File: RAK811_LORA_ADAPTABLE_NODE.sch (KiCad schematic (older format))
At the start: 32 parts, among them J1 Screw_Terminal_01x02, J10 Conn_01x01_Male, J11 Conn_01x01_Male, J12 Conn_01x01_Male, J13 Conn_01x01_Male, J14 Conn_01x01_Male, J15 Conn_01x01_Male, J16 Conn_01x01_Male, J17 Conn_01x01_Male, J18 Conn_01x01_Male, J19 Conn_01x01_Male, J2 Screw_Terminal_01x03, J20 Conn_01x01_Male, J21 Conn_01x01_Male, J22 Conn_01x01_Male, J23 Conn_01x01_Male, J3 Conn_01x01_Male, J4 Conn_01x01_Male, J5 Conn_01x01_Male, J6 Conn_01x01_Male, J7 Conn_Coaxial, J8 Conn_01x01_Male, J9 Conn_01x01_Male, U1 RAK811-HF

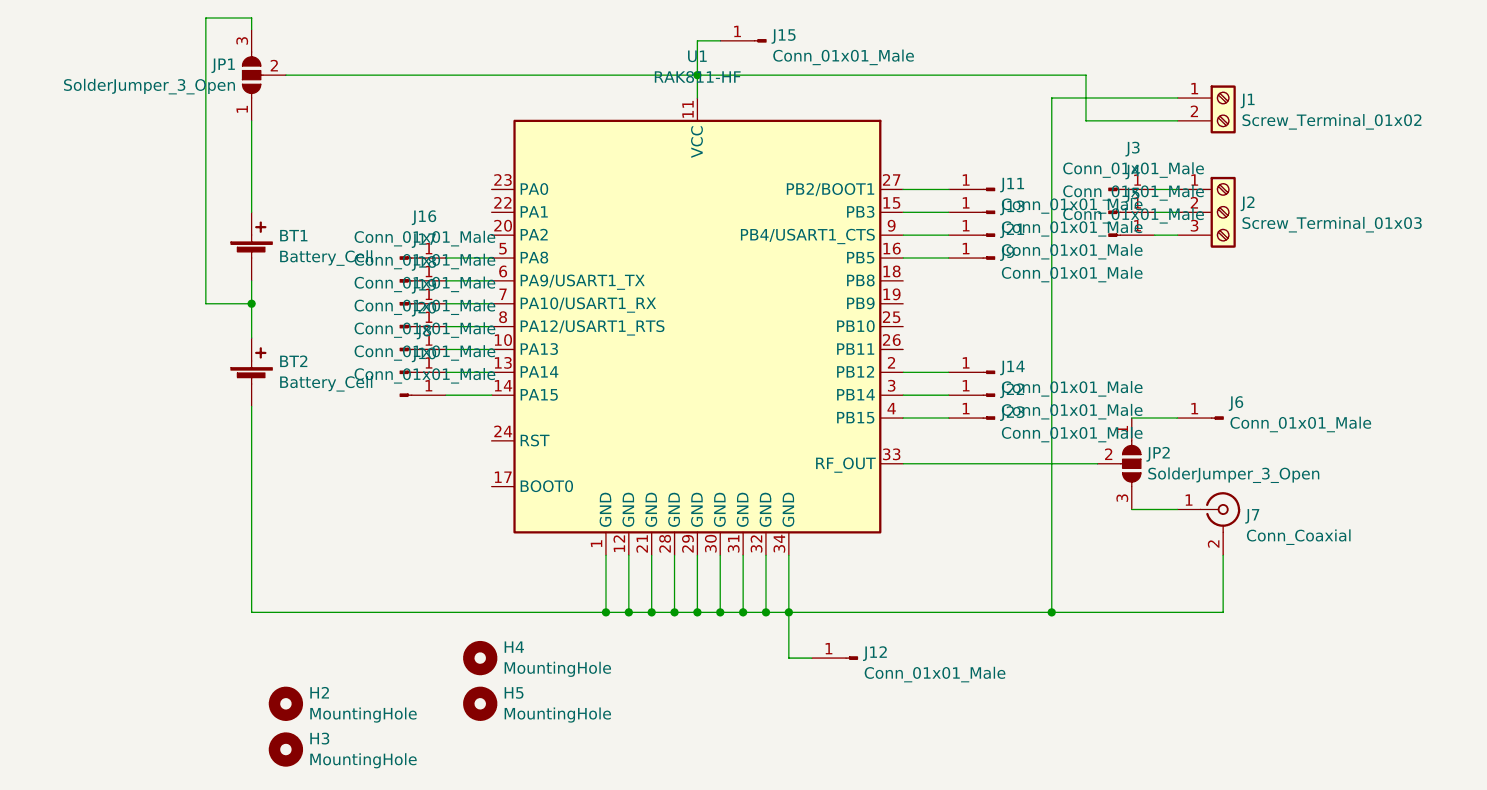
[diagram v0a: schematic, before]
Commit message: all i/o pins layout
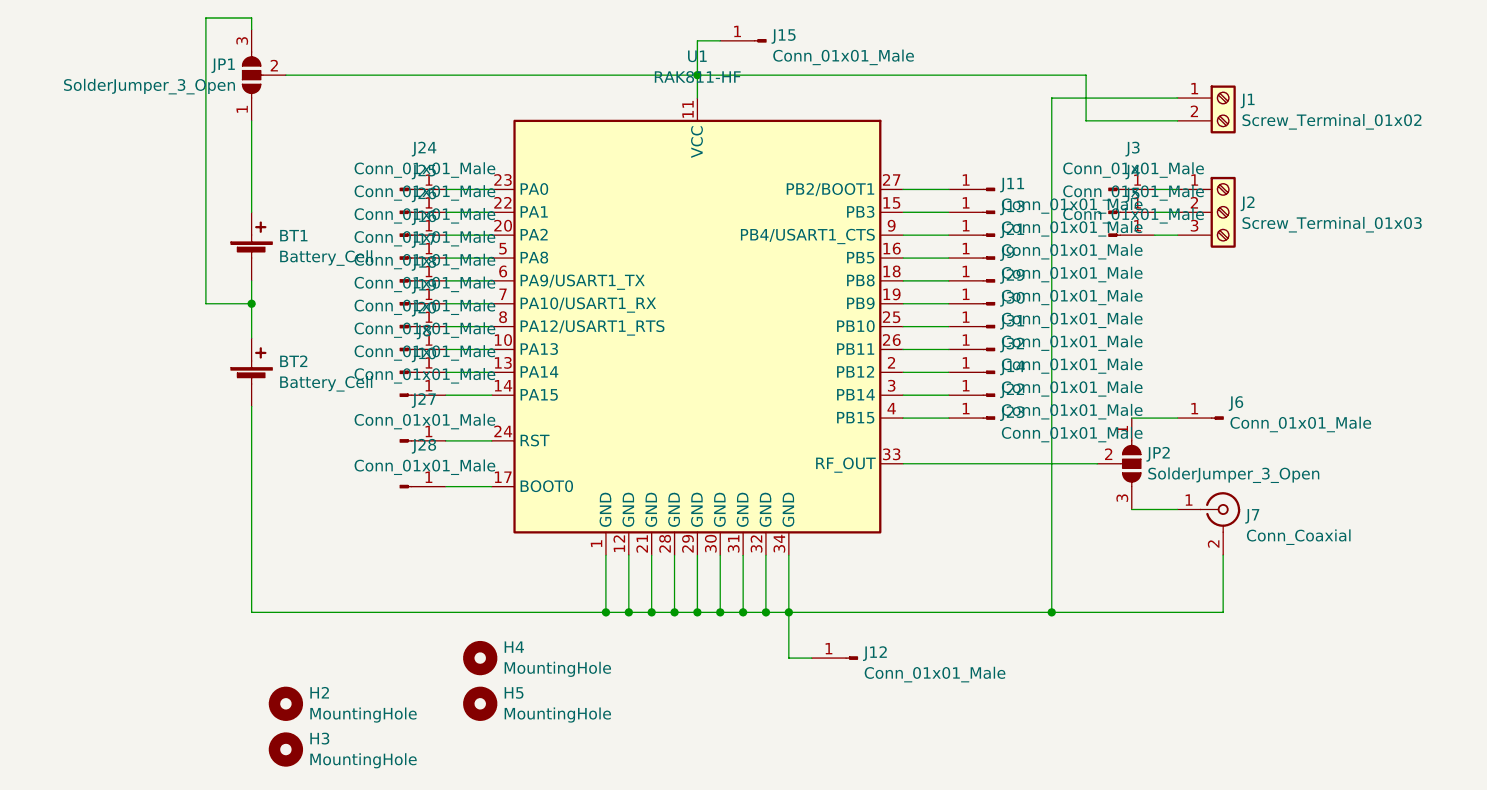
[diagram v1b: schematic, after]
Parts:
- added J24, J25, J26, J27, J28, J29, J30, J31, J32: Conn_01x01_Male, Connector_Wire:SolderWirePad_1x01_Drill0.8mm, symbol Connector:Conn_01x01_Male
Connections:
- net at U1.17 (BOOT0): now also J28.1 (Pin_1)
- net at U1.18 (PB8): now also J29.1 (Pin_1)
- net at U1.19 (PB9): now also J30.1 (Pin_1)
- net at U1.20 (PA2): now also J26.1 (Pin_1)
- net at U1.22 (PA1): now also J25.1 (Pin_1)
- net at U1.23 (PA0): now also J24.1 (Pin_1)
- net at U1.24 (RST): now also J27.1 (Pin_1)
- net at U1.25 (PB10): now also J31.1 (Pin_1)
- net at U1.26 (PB11): now also J32.1 (Pin_1)
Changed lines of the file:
@@
 Wire Wire Line
 	4350 3050 4550 3050
+$Comp
+L Connector:Conn_01x01_Male J26
+U 1 1 5EF46CC4
+P 4150 2550
+F 0 "J26" H 4258 2731 50  0000 C CNN
+F 1 "Conn_01x01_Male" H 4258 2640 50  0000 C CNN
+F 2 "Connector_Wire:SolderWirePad_1x01_Drill0.8mm" H 4150 2550 50  0001 C CNN
+F 3 "~" H 4150 2550 50  0001 C CNN
+	1    4150 2550
+	1    0    0    -1
+$EndComp
+$Comp
+L Connector:Conn_01x01_Male J25
+U 1 1 5EF4A3F0
+P 4150 2450
+F 0 "J25" H 4258 2631 50  0000 C CNN
+F 1 "Conn_01x01_Male" H 4258 2540 50  0000 C CNN
+F 2 "Connector_Wire:SolderWirePad_1x01_Drill0.8mm" H 4150 2450 50  0001 C CNN
+F 3 "~" H 4150 2450 50  0001 C CNN
+	1    4150 2450
+	1    0    0    -1
+$EndComp
+$Comp
+L Connector:Conn_01x01_Male J24
+U 1 1 5EF4DB52
+P 4150 2350
+F 0 "J24" H 4258 2531 50  0000 C CNN
+F 1 "Conn_01x01_Male" H 4258 2440 50  0000 C CNN
+F 2 "Connector_Wire:SolderWirePad_1x01_Drill0.8mm" H 4150 2350 50  0001 C CNN
+F 3 "~" H 4150 2350 50  0001 C CNN
+	1    4150 2350
+	1    0    0    -1
+$EndComp
+$Comp
+L Connector:Conn_01x01_Male J27
+U 1 1 5EF4EB2E
+P 4150 3450
+F 0 "J27" H 4258 3631 50  0000 C CNN
+F 1 "Conn_01x01_Male" H 4258 3540 50  0000 C CNN
+F 2 "Connector_Wire:SolderWirePad_1x01_Drill0.8mm" H 4150 3450 50  0001 C CNN
+F 3 "~" H 4150 3450 50  0001 C CNN
+	1    4150 3450
+	1    0    0    -1
+$EndComp
+$Comp
+L Connector:Conn_01x01_Male J28
+U 1 1 5EF4F1F7
+P 4150 3650
+F 0 "J28" H 4258 3831 50  0000 C CNN
+F 1 "Conn_01x01_Male" H 4258 3740 50  0000 C CNN
+F 2 "Connector_Wire:SolderWirePad_1x01_Drill0.8mm" H 4150 3650 50  0001 C CNN
+F 3 "~" H 4150 3650 50  0001 C CNN
+	1    4150 3650
+	1    0    0    -1
+$EndComp
+$Comp
+L Connector:Conn_01x01_Male J29
+U 1 1 5EF50306
+P 6750 2750
+F 0 "J29" H 6722 2774 50  0000 R CNN
+F 1 "Conn_01x01_Male" H 6722 2683 50  0000 R CNN
+F 2 "Connector_Wire:SolderWirePad_1x01_Drill0.8mm" H 6750 2750 50  0001 C CNN
+F 3 "~" H 6750 2750 50  0001 C CNN
+	1    6750 2750
+	-1   0    0    -1
+$EndComp
+$Comp
+L Connector:Conn_01x01_Male J30
+U 1 1 5EF5185E
+P 6750 2850
+F 0 "J30" H 6722 2874 50  0000 R CNN
+F 1 "Conn_01x01_Male" H 6722 2783 50  0000 R CNN
+F 2 "Connector_Wire:SolderWirePad_1x01_Drill0.8mm" H 6750 2850 50  0001 C CNN
+F 3 "~" H 6750 2850 50  0001 C CNN
+	1    6750 2850
+	-1   0    0    -1
+$EndComp
+$Comp
+L Connector:Conn_01x01_Male J31
+U 1 1 5EF52224
+P 6750 2950
+F 0 "J31" H 6722 2974 50  0000 R CNN
+F 1 "Conn_01x01_Male" H 6722 2883 50  0000 R CNN
+F 2 "Connector_Wire:SolderWirePad_1x01_Drill0.8mm" H 6750 2950 50  0001 C CNN
+F 3 "~" H 6750 2950 50  0001 C CNN
+	1    6750 2950
+	-1   0    0    -1
+$EndComp
+$Comp
+L Connector:Conn_01x01_Male J32
+U 1 1 5EF527FE
+P 6750 3050
+F 0 "J32" H 6722 3074 50  0000 R CNN
+F 1 "Conn_01x01_Male" H 6722 2983 50  0000 R CNN
+F 2 "Connector_Wire:SolderWirePad_1x01_Drill0.8mm" H 6750 3050 50  0001 C CNN
+F 3 "~" H 6750 3050 50  0001 C CNN
+	1    6750 3050
+	-1   0    0    -1
+$EndComp
+Wire Wire Line
+	4350 2550 4550 2550
+Wire Wire Line
+	4350 2450 4550 2450
+Wire Wire Line
+	4350 2350 4550 2350
+Wire Wire Line
+	4350 3450 4550 3450
+Wire Wire Line
+	4350 3650 4550 3650
+Wire Wire Line
+	6350 2750 6550 2750
+Wire Wire Line
+	6350 2850 6550 2850
+Wire Wire Line
+	6350 2950 6550 2950
+Wire Wire Line
+	6350 3050 6550 3050
 $EndSCHEMATC
